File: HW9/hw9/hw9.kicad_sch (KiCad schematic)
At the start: 33 parts, among them J1 Barrel_Jack_MountingPin, Q1 BC337, SW1 SW_MEC_5G, U1 LM317, U2 NE555P, U3 NE555P

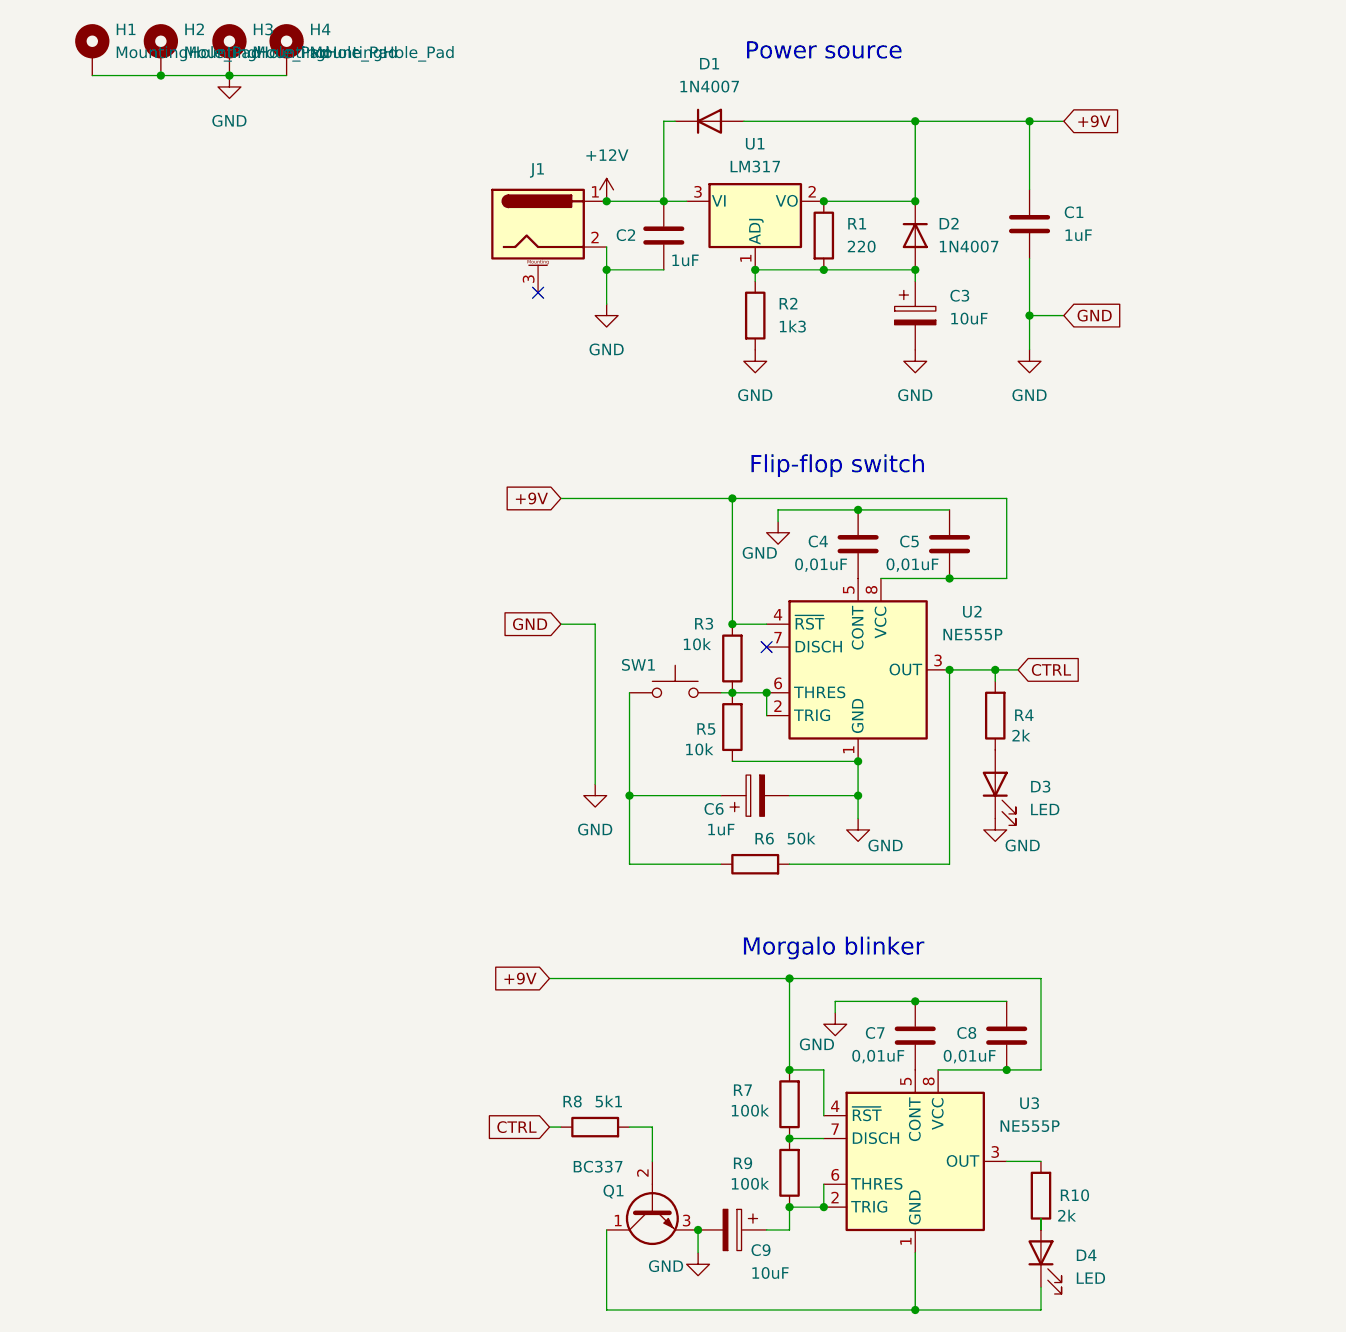
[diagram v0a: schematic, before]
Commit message: hw9 done
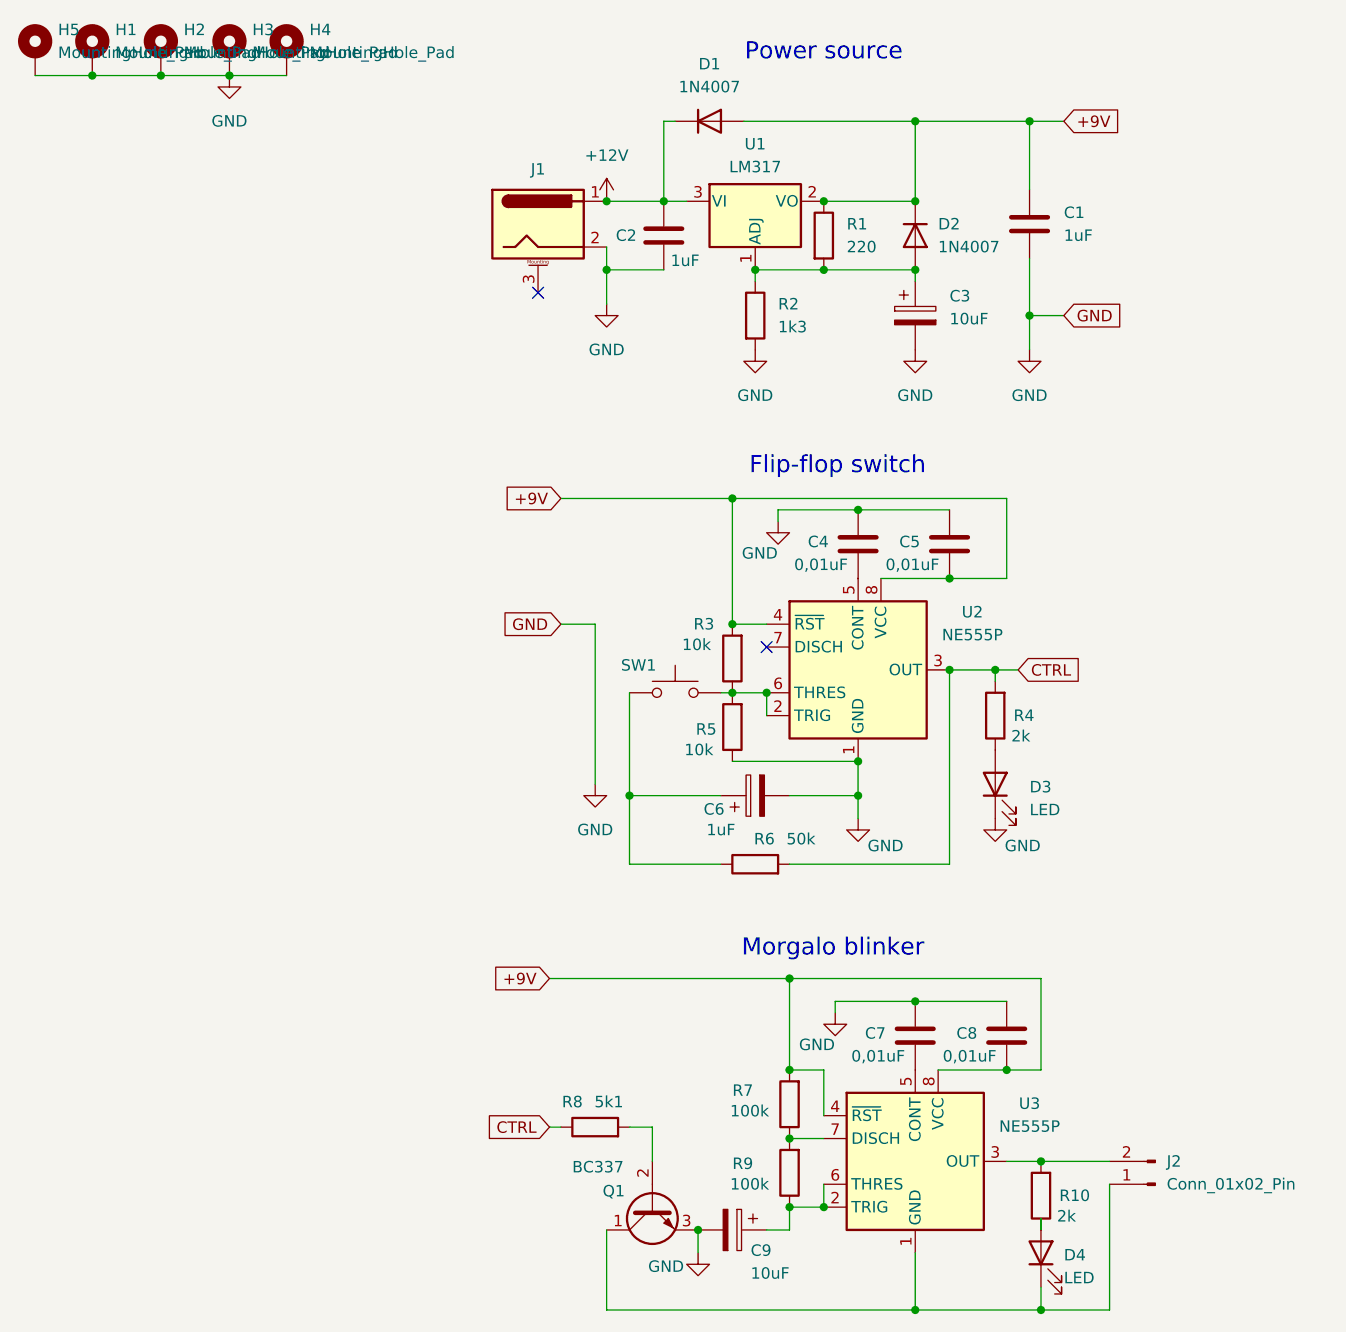
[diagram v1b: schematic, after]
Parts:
- added H5: MountingHole_Pad, MountingHole:MountingHole_2.2mm_M2_DIN965_Pad, symbol Mechanical:MountingHole_Pad
- added J2: Conn_01x02_Pin, Connector_Molex:Molex_PicoBlade_53261-0271_1x02-1MP_P1.25mm_Horizontal, symbol Connector:Conn_01x02_Pin
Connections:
- net GND: now also H5.1
- net at D4.1 (K), Q1.1 (C), U3.1 (GND): now also J2.1 (Pin_1)
- net at R10.2, U3.3 (OUT): now also J2.2 (Pin_2)
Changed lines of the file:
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@@
+	)
+	(junction
+		(at 129.54 170.18)
+		(diameter 0)
+		(color 0 0 0 0)
 	)
 	(junction
@@
 	)
 	(junction
+		(at 129.54 153.67)
+		(diameter 0)
+		(color 0 0 0 0)
+	)
+	(junction
 		(at 124.46 99.06)
+		(diameter 0)
+		(color 0 0 0 0)
+	)
+	(junction
+		(at 24.13 33.02)
 		(diameter 0)
 		(color 0 0 0 0)
@@
 	(wire
 		(pts
+			(xy 137.16 156.21) (xy 137.16 170.18)
+		)
+		(stroke
+			(width 0)
+			(type default)
+		)
+	)
+	(wire
+		(pts
 			(xy 81.28 54.61) (xy 87.63 54.61)
 		)
@@
 	(wire
 		(pts
+			(xy 129.54 153.67) (xy 137.16 153.67)
+		)
+		(stroke
+			(width 0)
+			(type default)
+		)
+	)
+	(wire
+		(pts
+			(xy 17.78 33.02) (xy 24.13 33.02)
+		)
+		(stroke
+			(width 0)
+			(type default)
+		)
+	)
+	(wire
+		(pts
 			(xy 115.57 163.83) (xy 115.57 170.18)
 		)
@@
 		(pts
 			(xy 81.28 46.99) (xy 87.63 46.99)
+		)
+		(stroke
+			(width 0)
+			(type default)
+		)
+	)
+	(wire
+		(pts
+			(xy 137.16 170.18) (xy 129.54 170.18)
 		)
 		(stroke
@@
 		(on_board yes)
 		(dnp no)
-		(fields_autoplaced yes)
 		(property "Reference" "D4"
-			(at 133.35 164.1474 90)
+			(at 132.08 164.084 90)
 			(effects
 				(font
@@
 		)
 		(property "Value" "LED"
-			(at 133.35 166.6874 90)
+			(at 132.08 166.624 90)
 			(effects
 				(font
@@
 				(path "/e4439f26-5216-4c4c-b757-2121e723fa89"
 					(reference "SW1")
+					(unit 1)
+				)
+			)
+		)
+	)
+	(symbol
+		(lib_id "Mechanical:MountingHole_Pad")
+		(at 17.78 30.48 0)
+		(unit 1)
+		(exclude_from_sim no)
+		(in_bom no)
+		(on_board yes)
+		(dnp no)
+		(fields_autoplaced yes)
+		(property "Reference" "H5"
+			(at 20.32 27.9399 0)
+			(effects
+				(font
+					(size 1.27 1.27)
+				)
+				(justify left)
+			)
+		)
+		(property "Value" "MountingHole_Pad"
+			(at 20.32 30.4799 0)
+			(effects
+				(font
+					(size 1.27 1.27)
+				)
+				(justify left)
+			)
+		)
+		(property "Footprint" "MountingHole:MountingHole_2.2mm_M2_DIN965_Pad"
+			(at 17.78 30.48 0)
+			(effects
+				(font
+					(size 1.27 1.27)
+				)
+				(hide yes)
+			)
+		)
+		(property "Datasheet" "~"
+			(at 17.78 30.48 0)
+			(effects
+				(font
+					(size 1.27 1.27)
+				)
+				(hide yes)
+			)
+		)
+		(property "Description" "Mounting Hole with connection"
+			(at 17.78 30.48 0)
+			(effects
+				(font
+					(size 1.27 1.27)
+				)
+				(hide yes)
+			)
+		)
+		(pin "1"
+		)
+		(instances
+			(project "hw9"
+				(path "/e4439f26-5216-4c4c-b757-2121e723fa89"
+					(reference "H5")
 					(unit 1)
 				)
@@
 					(unit 1)
 				)
+			)
+		)
+	)
+	(symbol
+		(lib_id "Connector:Conn_01x02_Pin")
+		(at 142.24 156.21 180)
+		(unit 1)
+		(exclude_from_sim no)
+		(in_bom yes)
+		(on_board yes)
+		(dnp no)
+		(fields_autoplaced yes)
+		(property "Reference" "J2"
+			(at 143.51 153.6699 0)
+			(effects
+				(font
+					(size 1.27 1.27)
+				)
+				(justify right)
+			)
+		)
+		(property "Value" "Conn_01x02_Pin"
+			(at 143.51 156.2099 0)
+			(effects
+				(font
+					(size 1.27 1.27)
+				)
+				(justify right)
+			)
+		)
+		(property "Footprint" "Connector_Molex:Molex_PicoBlade_53261-0271_1x02-1MP_P1.25mm_Horizontal"
+			(at 142.24 156.21 0)
+			(effects
+				(font
+					(size 1.27 1.27)
+				)
+				(hide yes)
+			)
+		)
+		(property "Datasheet" "~"
+			(at 142.24 156.21 0)
+			(effects
+				(font
+					(size 1.27 1.27)
+				)
+				(hide yes)
+			)
+		)
+		(property "Description" "Generic connector, single row, 01x02, script generated"
+			(at 142.24 156.21 0)
+			(effects
+				(font
+					(size 1.27 1.27)
+				)
+				(hide yes)
+			)
+		)
+		(pin "2"
+		)
+		(pin "1"
+		)
+		(instances
+			(project ""
+				(path "/e4439f26-5216-4c4c-b757-2121e723fa89"
+					(reference "J2")
+					(unit 1)
+				)
